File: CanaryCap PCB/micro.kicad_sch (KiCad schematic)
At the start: 23 parts, among them SW1 SW_MEC_5E, SW2 SW_MEC_5E, SW3 SW_MEC_5E, U3 ESP32-C6FH4

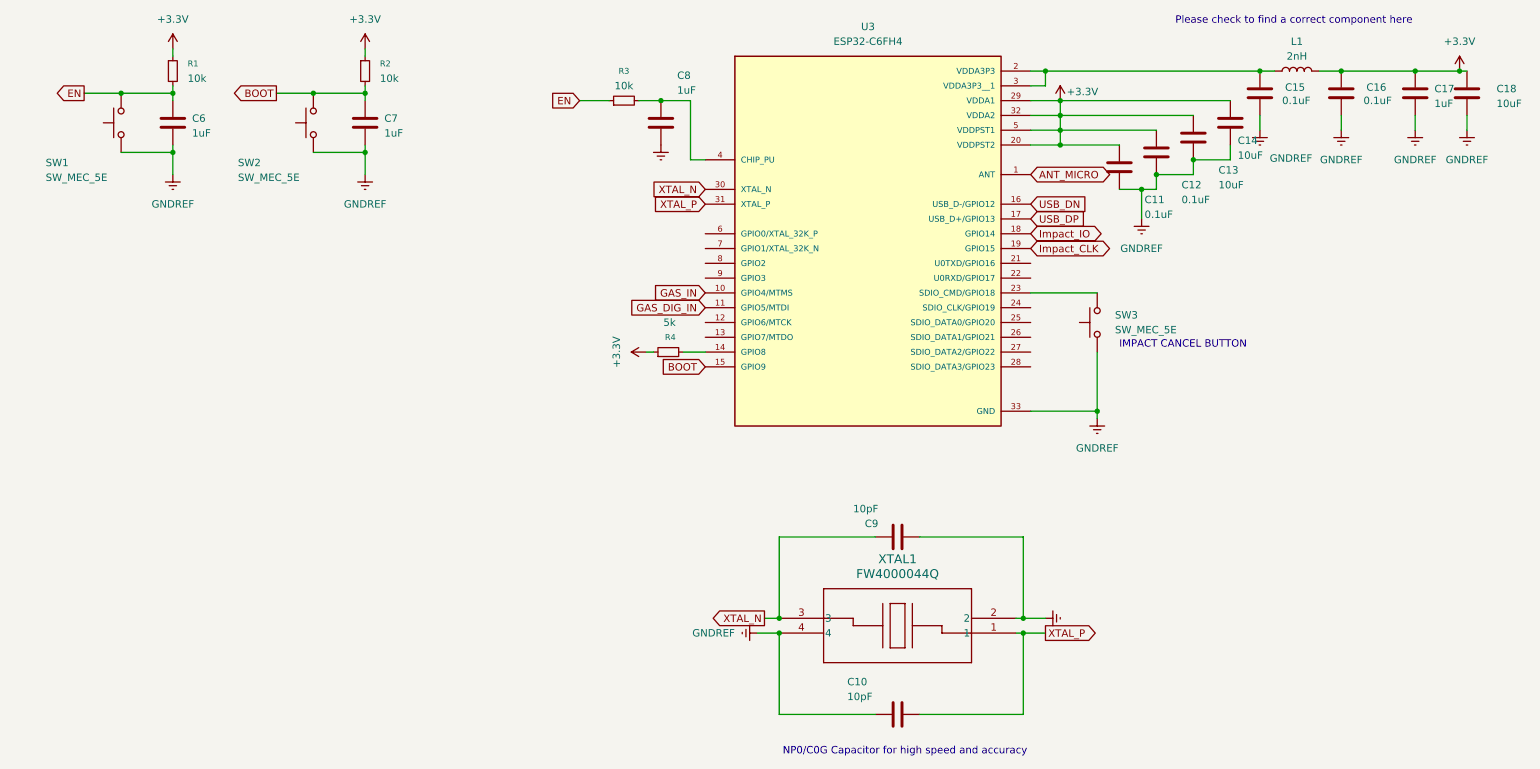
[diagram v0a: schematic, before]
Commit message: Finished level for packaging
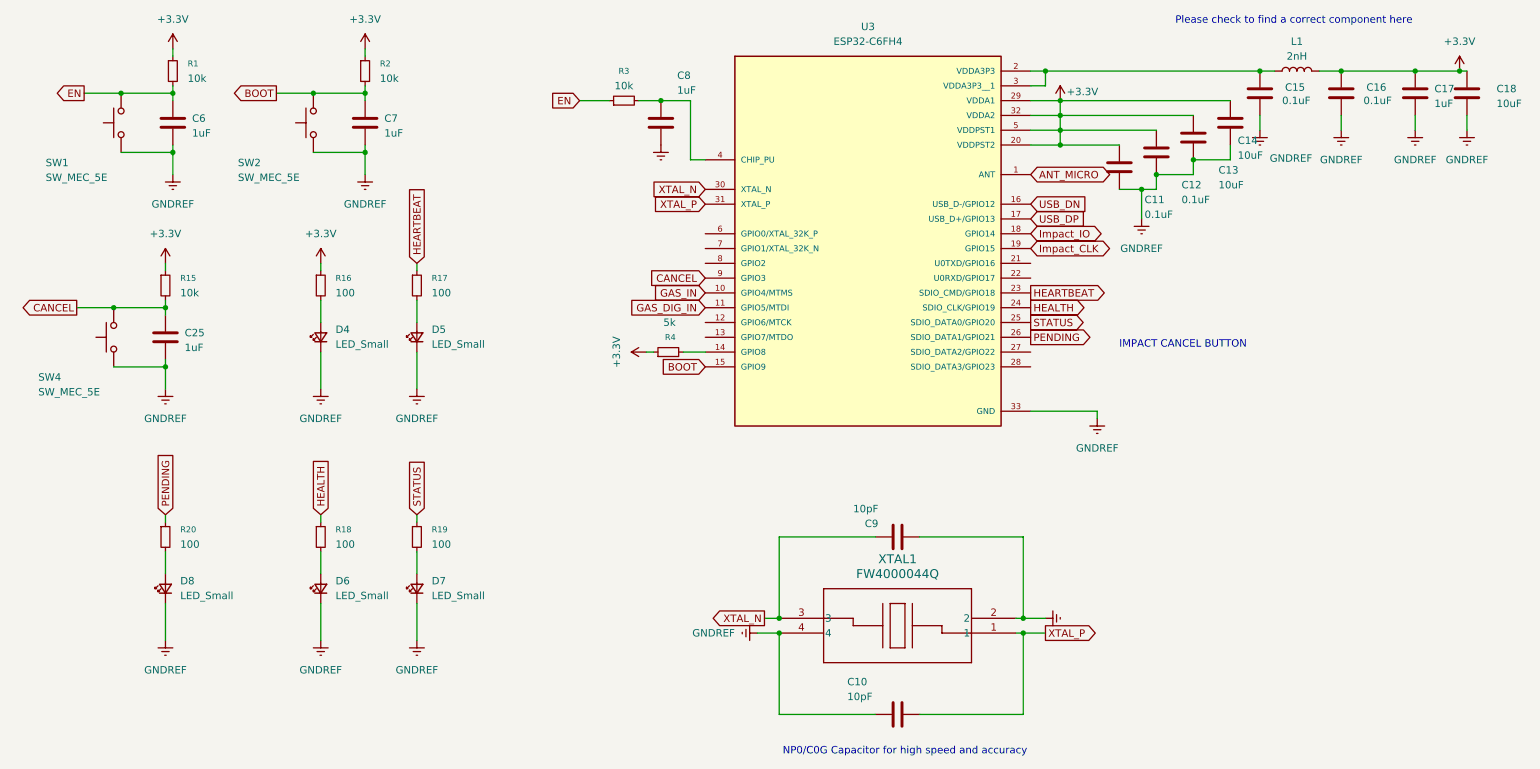
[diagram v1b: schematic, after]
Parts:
- removed SW3: SW_MEC_5E, Button_Switch_SMD:SW_SPST_EVQP2_MiddlePushTravel_H2.5mm, symbol Switch:SW_Push
- added C25: 1uF, Capacitor_SMD:C_0603_1608Metric_Pad1.08x0.95mm_HandSolder, symbol Device:C
- added D4, D5, D6, D7, D8: LED_Small, LED_SMD:LED_0603_1608Metric_Pad1.05x0.95mm_HandSolder, symbol Device:LED_Small
- added R15: 10k, Resistor_SMD:R_0603_1608Metric_Pad0.98x0.95mm_HandSolder, symbol Device:R_Small
- added R16, R17, R18, R19, R20: 100, Resistor_SMD:R_0603_1608Metric_Pad0.98x0.95mm_HandSolder, symbol Device:R_Small
- added SW4: SW_MEC_5E, Button_Switch_SMD:SW_SPST_EVQP2_MiddlePushTravel_H2.5mm, symbol Switch:SW_Push
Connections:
- net +3.3V: now also R15.1, R16.1
- net GNDREF: now also C25.2, D4.1 (K), D5.1 (K), D6.1 (K), D7.1 (K), D8.1 (K), SW4.1
- net HEARTBEAT: now reaches U3.23 (SDIO_CMD/GPIO18)
- net HEARTBEAT: now also R17.1
- net HEALTH: now reaches U3.24 (SDIO_CLK/GPIO19)
- net HEALTH: now also R18.1
- net STATUS: now reaches U3.25 (SDIO_DATA0/GPIO20)
- net STATUS: now also R19.1
- net PENDING: now reaches U3.26 (SDIO_DATA1/GPIO21)
- net PENDING: now also R20.1
- net CANCEL: now reaches U3.9 (GPIO3)
- net CANCEL: now also C25.1, R15.2, SW4.2
- new net: D5.2 (A), R17.2
- new net: D4.2 (A), R16.2
- new net: D6.2 (A), R18.2
- new net: D8.2 (A), R20.2
- new net: D7.2 (A), R19.2
